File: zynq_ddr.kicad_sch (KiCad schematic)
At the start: 91 parts, among them U6 XC7Z020-2CLG400I, U700 MT41K256M16TW-107 IT:P, U701 MT41K256M16TW-107 IT:P

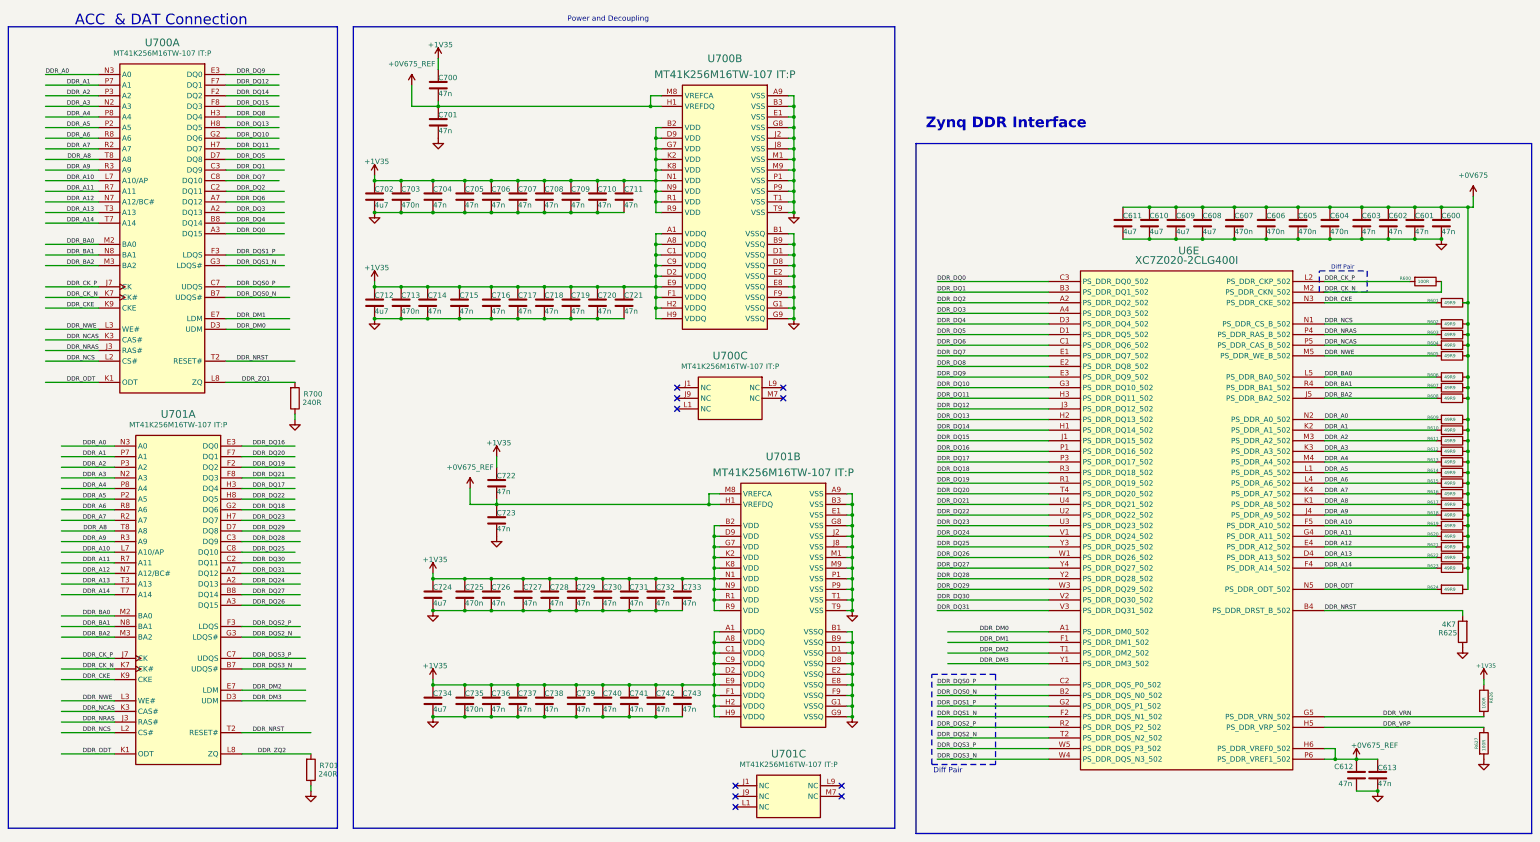
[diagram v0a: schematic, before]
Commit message: ram-zynq-updated
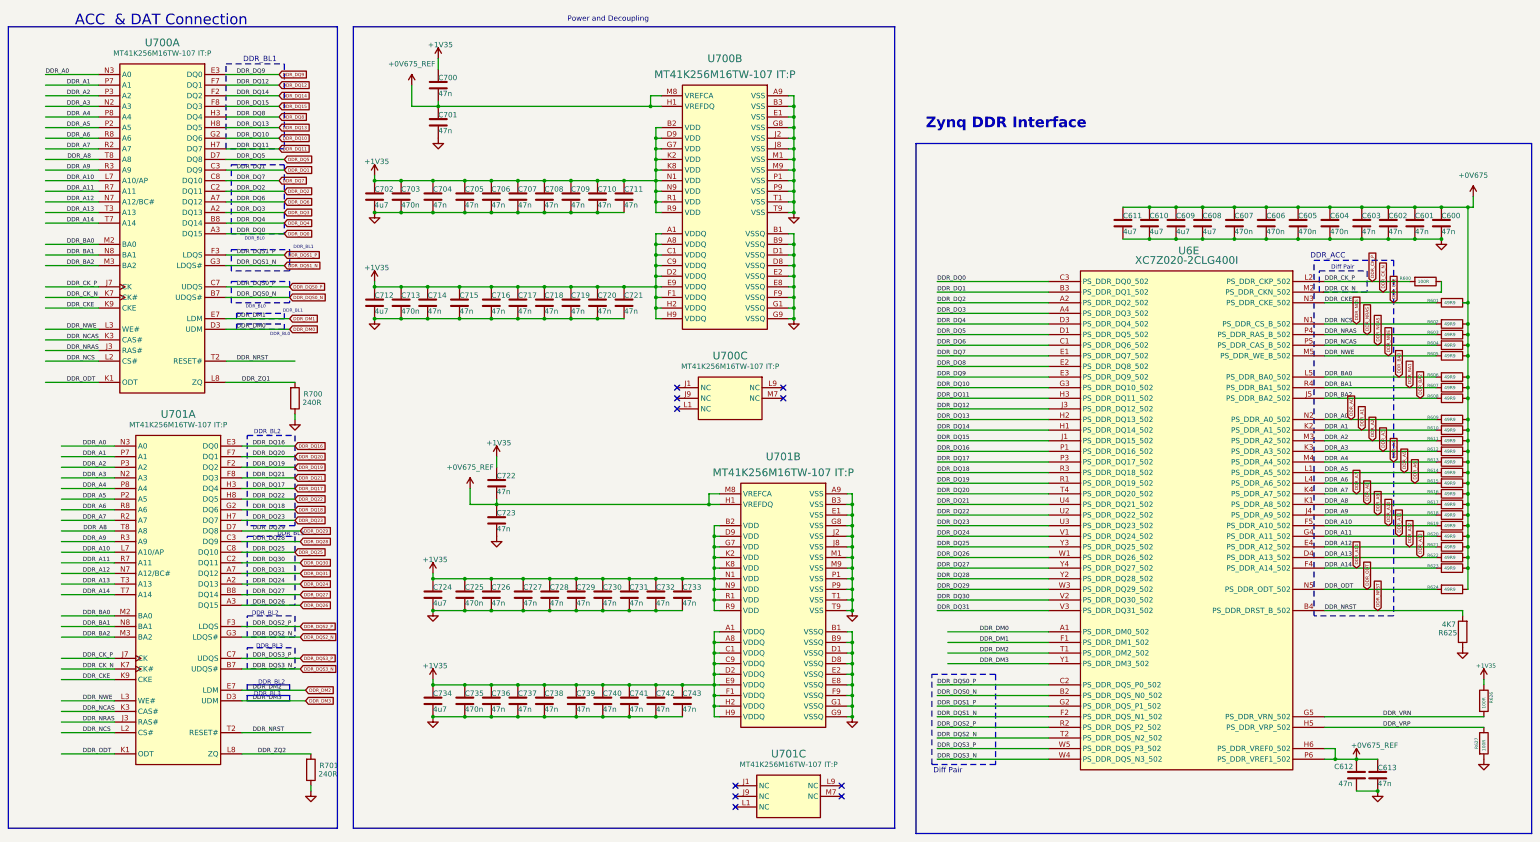
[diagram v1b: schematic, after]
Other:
- note added: "DDR_ACC"
- note added: "DDR_BL0"
- note added: "DDR_BL1"
- note added: "DDR_BL2"
- note added: "DDR_BL3"
